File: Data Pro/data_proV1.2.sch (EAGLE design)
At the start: 75 parts, among them CN1 DCIN, IC1 4049N, IC2 MCP3008, IC3 LM324D, IC4 MCP73871, IC6 AT24CP, J1 RASPBERRYPI-40-PIN-GPIO, J2 A2, J3 A3, J4 A4, J5 A1, J6 D1, J7 D2, J8 D3, J9 D4, U1 DS18B20, U2 TPS61200, X1 32.768khz

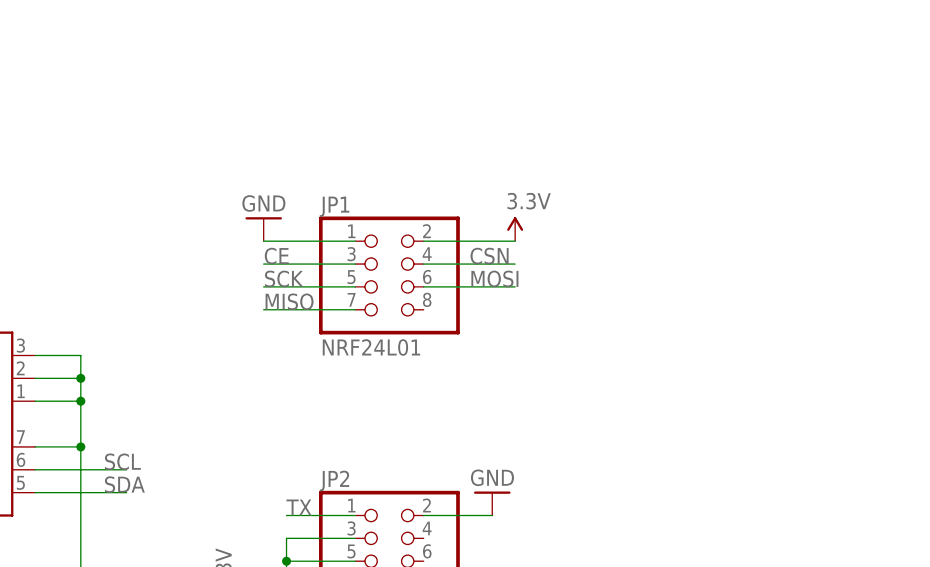
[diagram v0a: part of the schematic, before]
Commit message: Data pro complete
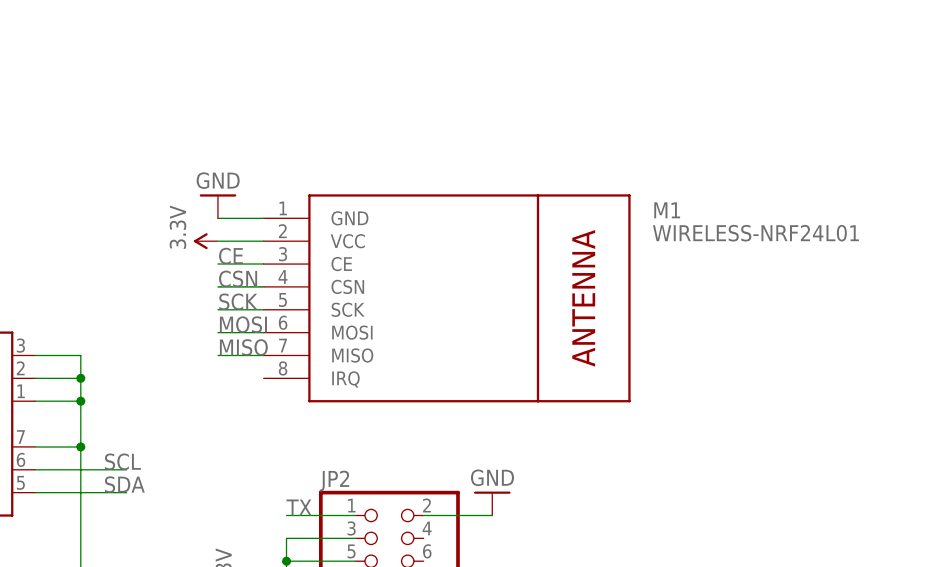
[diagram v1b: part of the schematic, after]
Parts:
- removed JP1: NRF24L01, pinhead:PINHD-2X4
- added M1: WIRELESS-NRF24L01, diy-modules:WIRELESS-NRF24L01
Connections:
- net 3.3V: now also M1.VCC; no longer JP1.2
- net CE: now also M1.CE; no longer JP1.3
- net CSN: now also M1.CSN; no longer JP1.4
- net GND: now also M1.GND; no longer JP1.1
- net MISO: now also M1.MISO; no longer JP1.7
- net MOSI: now also M1.MOSI; no longer JP1.6
- net SCK: now also M1.SCK; no longer JP1.5
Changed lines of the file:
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@@
 <part name="GND17" library="SparkFun-Aesthetics" deviceset="GND" device=""/>
 <part name="SUPPLY14" library="SparkFun-Aesthetics" deviceset="3.3V" device=""/>
-<part name="JP1" library="pinhead" deviceset="PINHD-2X4" device="" value="NRF24L01"/>
-<part name="GND18" library="SparkFun-Aesthetics" deviceset="GND" device=""/>
-<part name="SUPPLY15" library="SparkFun-Aesthetics" deviceset="3.3V" device=""/>
 <part name="U1" library="SparkFun-Sensors" deviceset="DS18B20" device=""/>
 <part name="SUPPLY16" library="SparkFun-Aesthetics" deviceset="3.3V" device=""/>
@@
 <part name="THERM" library="adafruit" deviceset="R-US_" device="FLIPFLOP" value="10K"/>
 <part name="GND39" library="SparkFun" deviceset="GND" device=""/>
+<part name="M1" library="diy-modules" deviceset="WIRELESS-NRF24L01" device=""/>
+<part name="SUPPLY24" library="SparkFun-Aesthetics" deviceset="3.3V" device=""/>
+<part name="GND31" library="SparkFun-Aesthetics" deviceset="GND" device=""/>
 </parts>
 <sheets>
@@
 <instance part="GND17" gate="1" x="259.08" y="76.2"/>
 <instance part="SUPPLY14" gate="G$1" x="269.24" y="88.9" rot="R270"/>
-<instance part="JP1" gate="A" x="299.72" y="142.24"/>
-<instance part="GND18" gate="1" x="287.02" y="149.86" rot="R180"/>
-<instance part="SUPPLY15" gate="G$1" x="314.96" y="147.32"/>
 <instance part="U1" gate="G$1" x="129.54" y="162.56"/>
 <instance part="SUPPLY16" gate="G$1" x="116.84" y="170.18" rot="R90"/>
@@
 <instance part="THERM" gate="G$1" x="274.32" y="-35.56" rot="R90"/>
 <instance part="GND39" gate="1" x="162.56" y="35.56" rot="R270"/>
+<instance part="M1" gate="G$1" x="309.88" y="139.7"/>
+<instance part="SUPPLY24" gate="G$1" x="281.94" y="147.32" rot="R90"/>
+<instance part="GND31" gate="1" x="281.94" y="152.4" rot="R180"/>
 </instances>
 <busses>
@@
 <wire x1="-15.24" y1="53.34" x2="-15.24" y2="58.42" width="0.1524" layer="91"/>
 <pinref part="GND10" gate="1" pin="GND"/>
-</segment>
-<segment>
-<pinref part="JP1" gate="A" pin="1"/>
-<wire x1="297.18" y1="147.32" x2="287.02" y2="147.32" width="0.1524" layer="91"/>
-<pinref part="GND18" gate="1" pin="GND"/>
 </segment>
 <segment>
@@
 <pinref part="THERM" gate="G$1" pin="1"/>
 </segment>
+<segment>
+<pinref part="M1" gate="G$1" pin="GND"/>
+<wire x1="287.02" y1="149.86" x2="281.94" y2="149.86" width="0.1524" layer="91"/>
+<pinref part="GND31" gate="1" pin="GND"/>
+</segment>
 </net>
 <net name="3.3V" class="0">
@@
 <pinref part="U$1" gate="G$1" pin="OUT"/>
 <wire x1="269.24" y1="88.9" x2="266.7" y2="88.9" width="0.1524" layer="91"/>
-</segment>
-<segment>
-<pinref part="JP1" gate="A" pin="2"/>
-<wire x1="304.8" y1="147.32" x2="314.96" y2="147.32" width="0.1524" layer="91"/>
-<pinref part="SUPPLY15" gate="G$1" pin="3.3V"/>
 </segment>
 <segment>
@@
 <junction x="289.56" y="111.76"/>
 <junction x="289.56" y="109.22"/>
+</segment>
+<segment>
+<pinref part="M1" gate="G$1" pin="VCC"/>
+<wire x1="287.02" y1="147.32" x2="281.94" y2="147.32" width="0.1524" layer="91"/>
+<pinref part="SUPPLY24" gate="G$1" pin="3.3V"/>
 </segment>
 </net>
@@
 <net name="MOSI" class="0">
 <segment>
-<pinref part="JP1" gate="A" pin="6"/>
-<wire x1="304.8" y1="142.24" x2="314.96" y2="142.24" width="0.1524" layer="91"/>
-<label x="309.88" y="142.24" size="1.778" layer="95"/>
-</segment>
-<segment>
 <pinref part="IC2" gate="G$1" pin="DIN"/>
 <wire x1="129.54" y1="121.92" x2="137.16" y2="121.92" width="0.1524" layer="91"/>
@@
 <junction x="137.16" y="71.12"/>
 </segment>
+<segment>
+<pinref part="M1" gate="G$1" pin="MOSI"/>
+<wire x1="287.02" y1="137.16" x2="281.94" y2="137.16" width="0.1524" layer="91"/>
+<label x="281.94" y="137.16" size="1.778" layer="95"/>
+</segment>
 </net>
 <net name="CSN" class="0">
-<segment>
-<pinref part="JP1" gate="A" pin="4"/>
-<wire x1="304.8" y1="144.78" x2="314.96" y2="144.78" width="0.1524" layer="91"/>
-<label x="309.88" y="144.78" size="1.778" layer="95"/>
-</segment>
 <segment>
 <pinref part="IC2" gate="G$1" pin="/CS"/>
@@
 <label x="137.16" y="68.58" size="1.778" layer="95"/>
 </segment>
+<segment>
+<pinref part="M1" gate="G$1" pin="CSN"/>
+<wire x1="287.02" y1="142.24" x2="281.94" y2="142.24" width="0.1524" layer="91"/>
+<label x="281.94" y="142.24" size="1.778" layer="95"/>
+</segment>
 </net>
 <net name="CE" class="0">
-<segment>
-<pinref part="JP1" gate="A" pin="3"/>
-<wire x1="297.18" y1="144.78" x2="287.02" y2="144.78" width="0.1524" layer="91"/>
-<label x="287.02" y="144.78" size="1.778" layer="95"/>
-</segment>
 <segment>
 <pinref part="J1" gate="G$1" pin="GP25"/>
 <wire x1="129.54" y1="45.72" x2="134.62" y2="45.72" width="0.1524" layer="91"/>
 <label x="132.08" y="45.72" size="1.778" layer="95"/>
+</segment>
+<segment>
+<pinref part="M1" gate="G$1" pin="CE"/>
+<wire x1="287.02" y1="144.78" x2="281.94" y2="144.78" width="0.1524" layer="91"/>
+<label x="281.94" y="144.78" size="1.778" layer="95"/>
 </segment>
 </net>
@@
 </net>
 <net name="SCK" class="0">
-<segment>
-<pinref part="JP1" gate="A" pin="5"/>
-<wire x1="297.18" y1="142.24" x2="287.02" y2="142.24" width="0.1524" layer="91"/>
-<label x="287.02" y="142.24" size="1.778" layer="95"/>
-</segment>
 <segment>
 <pinref part="IC2" gate="G$1" pin="CLK"/>
@@
 <junction x="142.24" y="76.2"/>
 </segment>
+<segment>
+<pinref part="M1" gate="G$1" pin="SCK"/>
+<wire x1="287.02" y1="139.7" x2="281.94" y2="139.7" width="0.1524" layer="91"/>
+<label x="281.94" y="139.7" size="1.778" layer="95"/>
+</segment>
 </net>
 <net name="MISO" class="0">
-<segment>
-<pinref part="JP1" gate="A" pin="7"/>
-<wire x1="297.18" y1="139.7" x2="287.02" y2="139.7" width="0.1524" layer="91"/>
-<label x="287.02" y="139.7" size="1.778" layer="95"/>
-</segment>
 <segment>
 <pinref part="IC2" gate="G$1" pin="DOUT"/>
@@
 <junction x="139.7" y="73.66"/>
 </segment>
-</net>
+<segment>
+<pinref part="M1" gate="G$1" pin="MISO"/>
+<wire x1="287.02" y1="134.62" x2="281.94" y2="134.62" width="0.1524" layer="91"/>
+<label x="281.94" y="134.62" size="1.778" layer="95"/>
+</segment>
+</net>
